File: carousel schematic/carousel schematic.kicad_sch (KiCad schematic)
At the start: 4 parts, among them J1 Raspberry_Pi_5, M1 Motor_Servo front door, M2 Motor_Servo back door

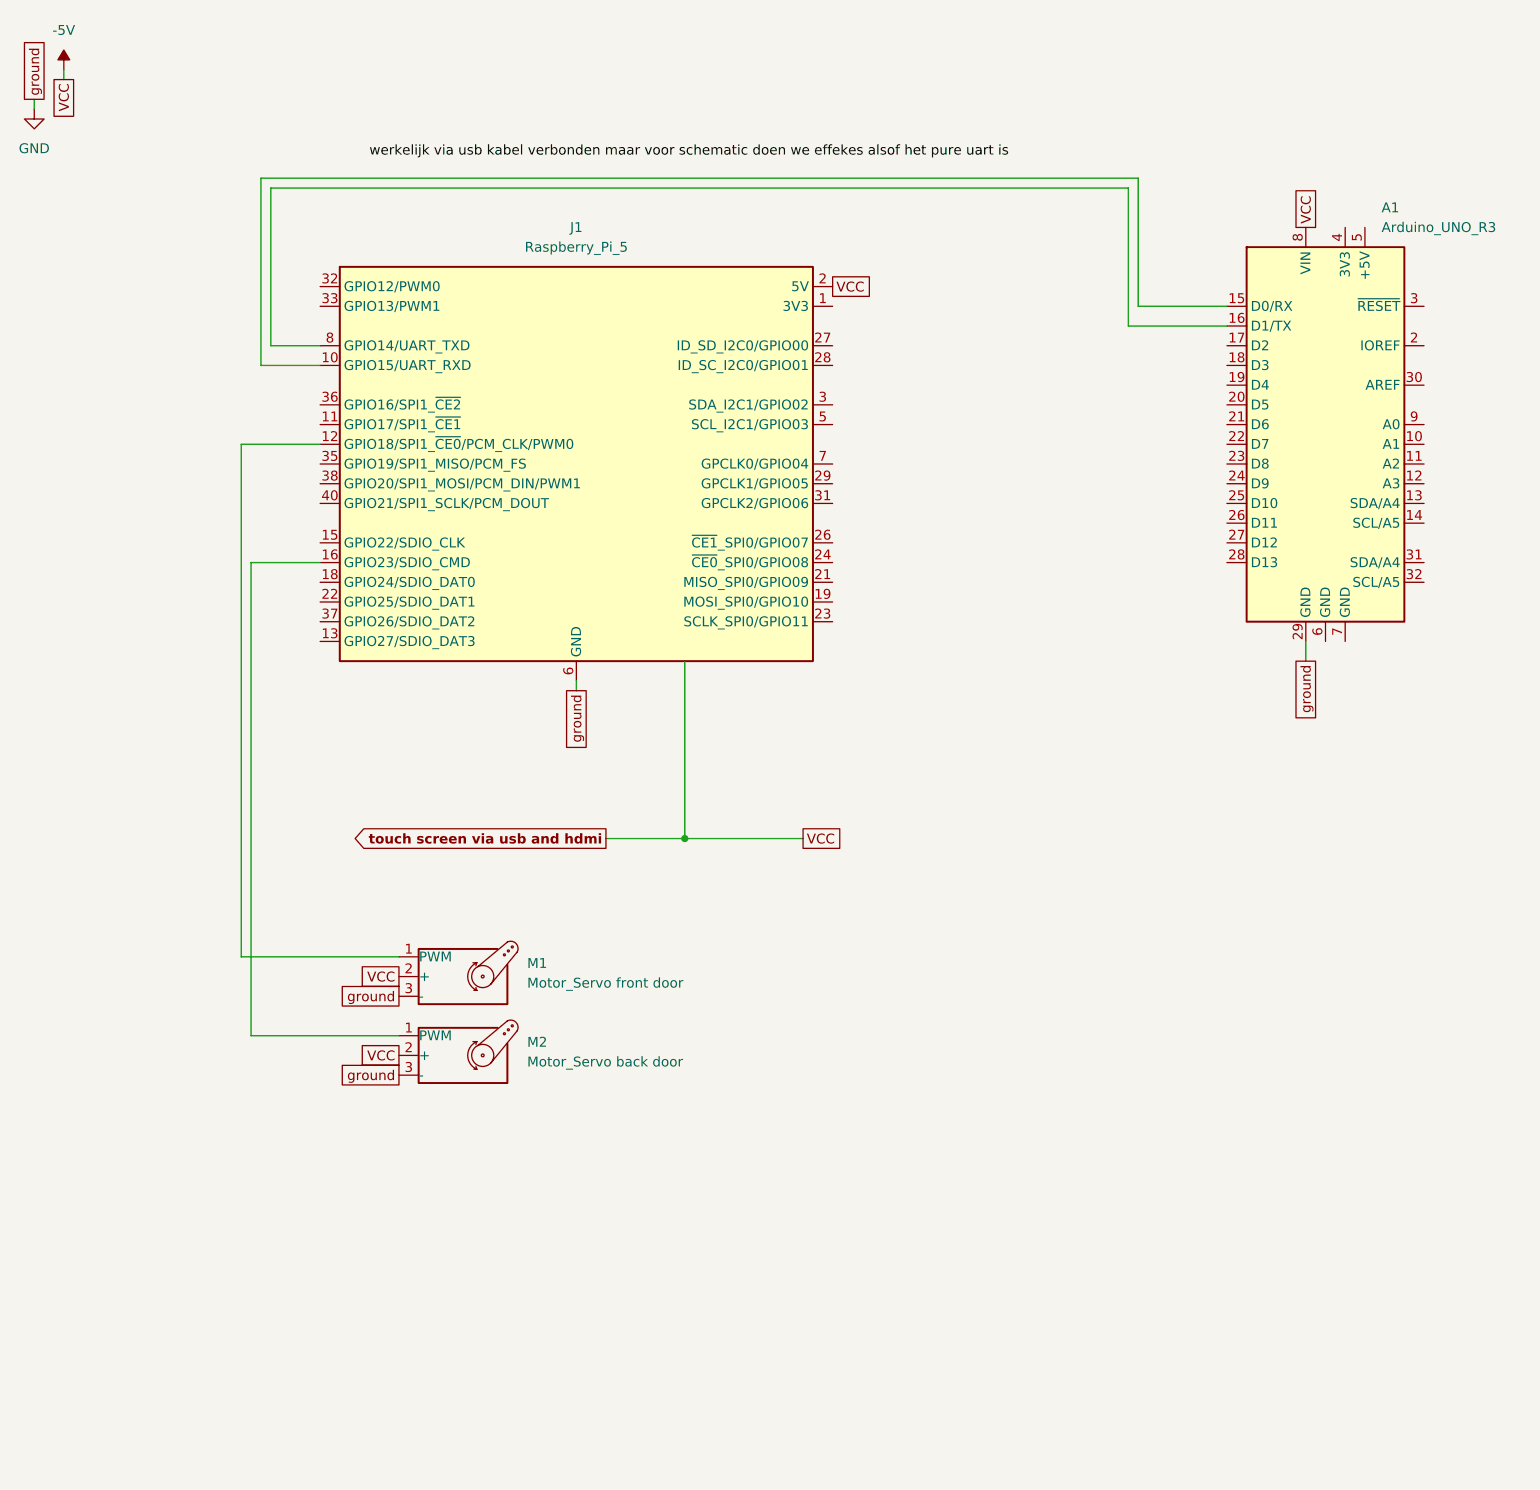
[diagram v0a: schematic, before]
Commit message: final schematic file
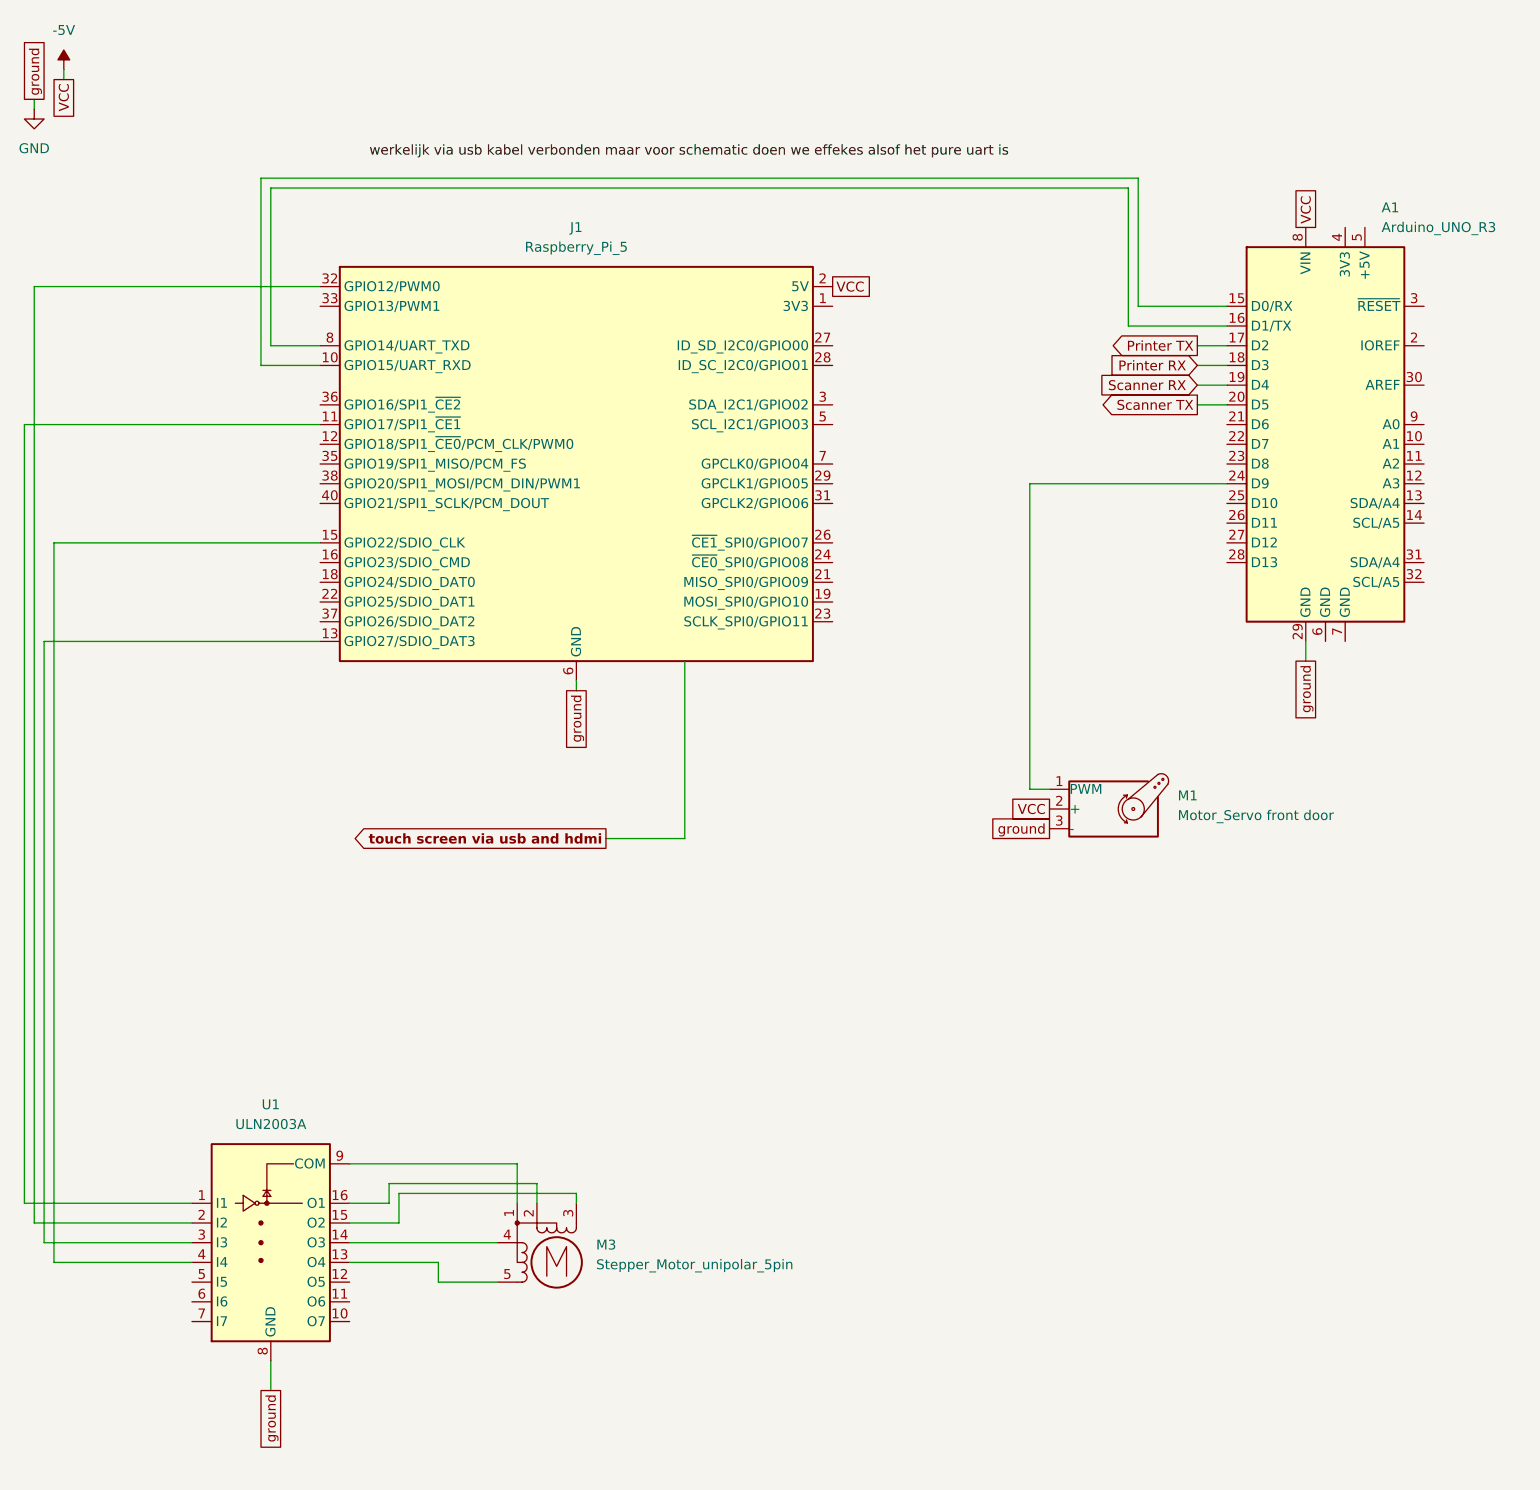
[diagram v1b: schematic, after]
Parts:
- removed M2: Motor_Servo back door, symbol Motor:Motor_Servo
- added M3: Stepper_Motor_unipolar_5pin, symbol Motor:Stepper_Motor_unipolar_5pin
- added U1: ULN2003A, symbol Transistor_Array:ULN2003A
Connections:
- net GND: now also U1.8 (GND)
- net at M1.1 (PWM): now also A1.24 (D9); no longer J1.12 (GPIO18/SPI1_~{CE0}/PCM_CLK/PWM0)
- net Printer TX: now reaches A1.17 (D2)
- net Printer RX: now reaches A1.18 (D3)
- net Scanner RX: now reaches A1.19 (D4)
- net Scanner TX: now reaches A1.20 (D5)
- net at J1.11 (GPIO17/SPI1_~{CE1}): now also U1.1 (I1)
- net at J1.13 (GPIO27/SDIO_DAT3): now also U1.3 (I3)
- net at J1.15 (GPIO22/SDIO_CLK): now also U1.4 (I4)
- net at J1.32 (GPIO12/PWM0): now also U1.2 (I2)
- new net: M3.1, U1.9 (COM)
- new net: M3.2, U1.16 (O1)
- new net: M3.3 (-), U1.15 (O2)
- new net: M3.4, U1.14 (O3)
- new net: M3.5, U1.13 (O4)
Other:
- moved on the sheet: M1

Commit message: update for last changes
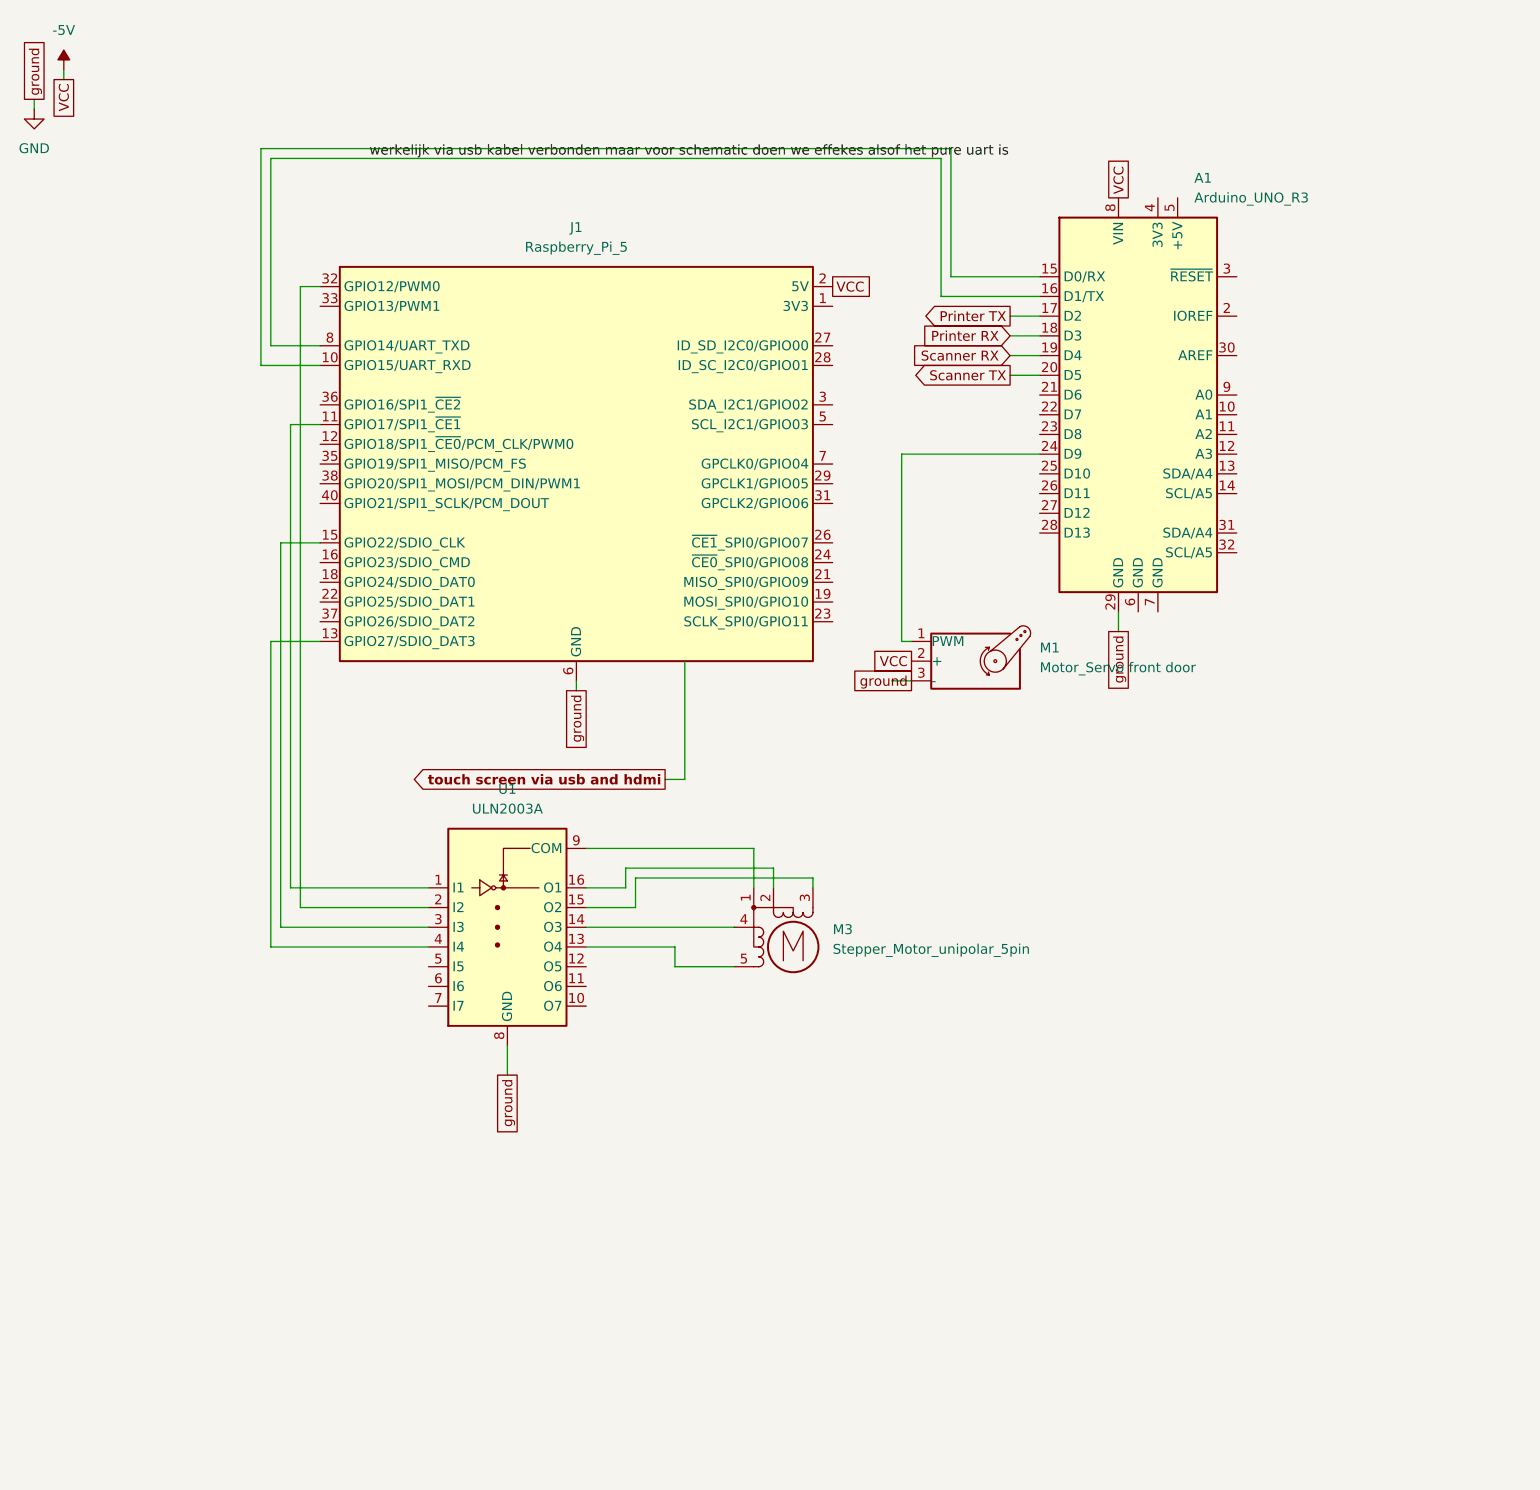
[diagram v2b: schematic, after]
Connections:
- net werkelijk via usb kabel verbonden maar voor schematic doen we effekes alsof het pure uart is: now also A1.16 (D1/TX), J1.8 (GPIO14/UART_TXD)
- net at J1.13 (GPIO27/SDIO_DAT3): now also U1.4 (I4); no longer U1.3 (I3)
- net at J1.15 (GPIO22/SDIO_CLK): now also U1.3 (I3); no longer U1.4 (I4)
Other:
- moved on the sheet: A1, M1, M3, U1
